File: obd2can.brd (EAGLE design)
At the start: 96.5 x 87.9 mm, 109 parts, among them IC1 SCANTOOL, IC3 LM339PWR, IC4 MCP2551, Q10 BSS138, Q1000 8MHz, Q3 MMBT2222, Q4 MMBT2222, Q7 ZXMP6A13FTA, Q8 MMBT2222, Q9 BSS138, SW1 6X3.5_TACT, U1 3.3V, U1000 SN65HVD235DR, U2 V_REG_317DPACK, U2000 STM32F072-LQFP48, U3 5V Reg., U3000 AP3211KTR-G1, X1000 RJ45_RIGHT_ANGLEMOLEX_95001-2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, X2 Male DB9, X2000 RJ45_RIGHT_ANGLEMOLEX_95001-2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, Y1 16MHz

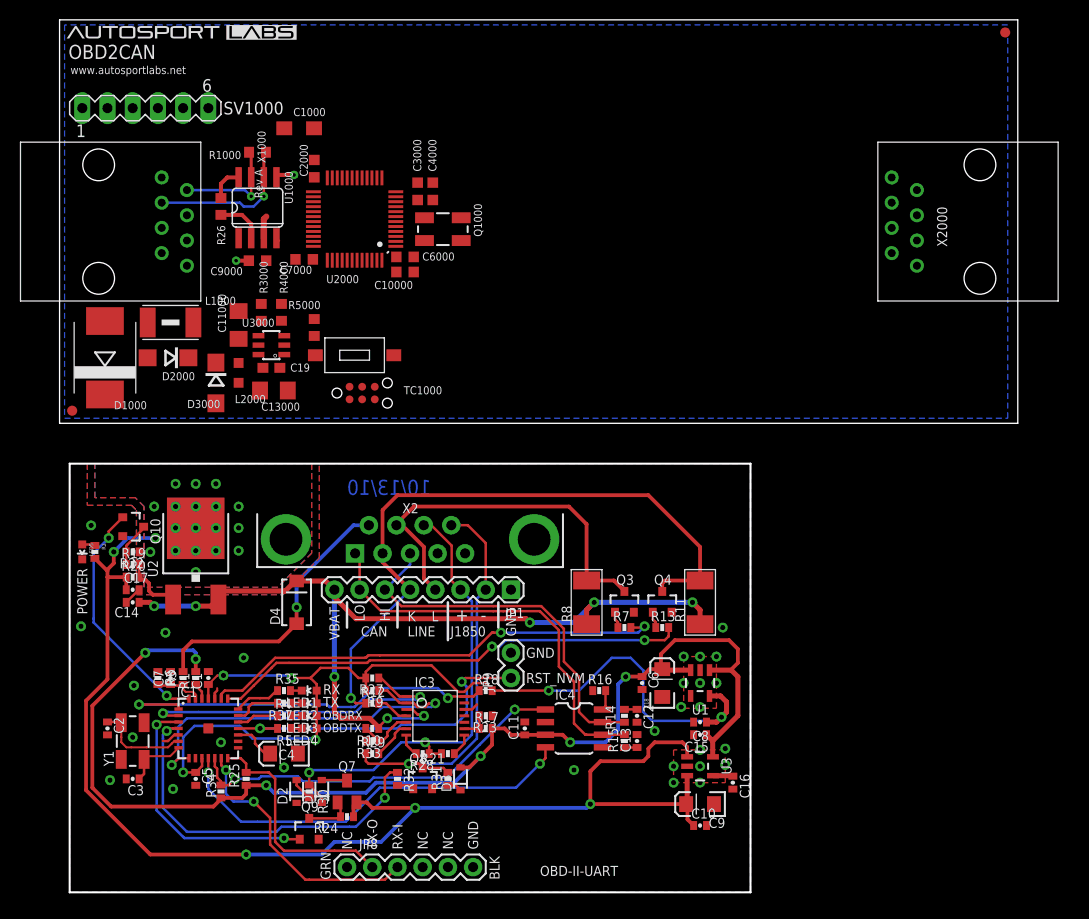
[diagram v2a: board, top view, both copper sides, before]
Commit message: label adjustment, snapshot image
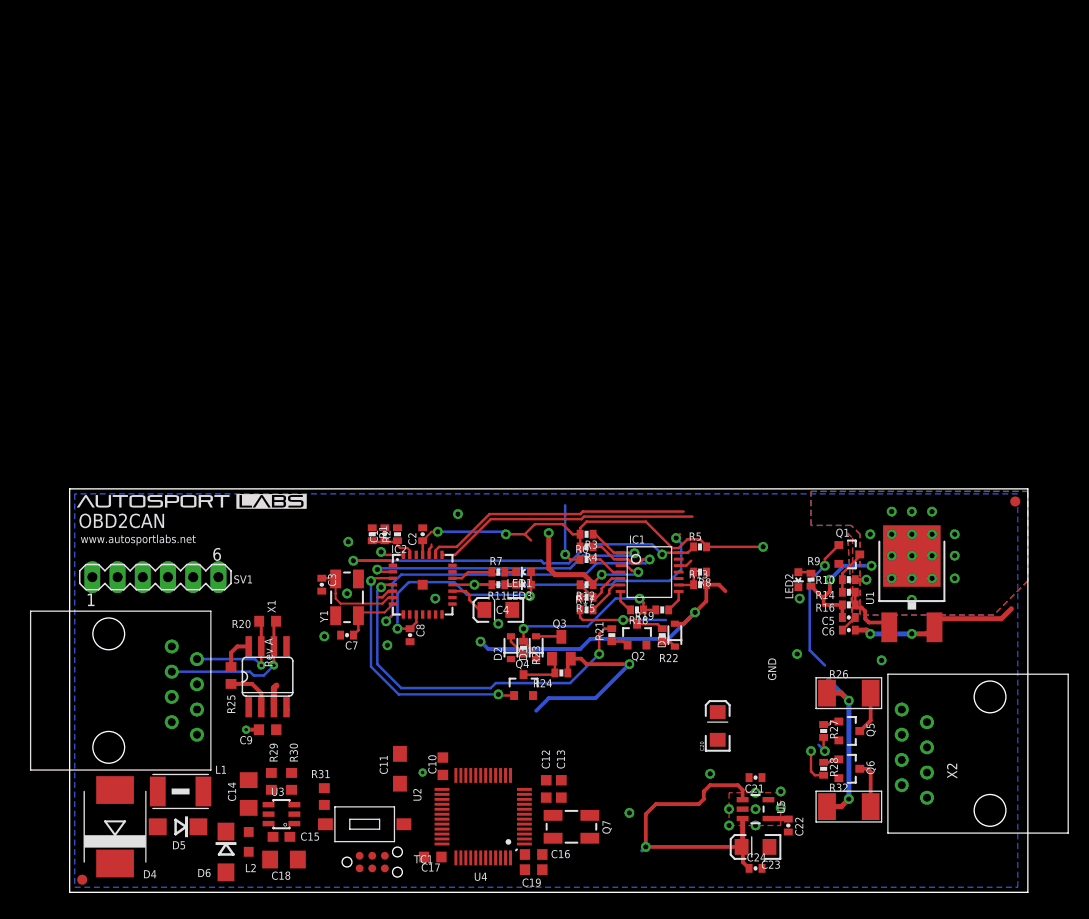
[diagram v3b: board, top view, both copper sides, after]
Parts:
- removed C1000: 10uF, rcl:SMC_A
- removed C10000: 1uf, rcl:C0603K
- removed C11000, C13000: 22uF, rcl:C1206
- removed C2000, C6000, C9000: 0.1uf, rcl:C0603K
- removed C3000, C7000: 4.7uf, rcl:C0603K
- removed C4000: 0.01uf, rcl:C0603K
- removed D1000: (no value), diode:SMC
- removed D2000: 400V 1A, smt_diodes:SMA
- removed D3000: SCHOTTKY, smt_diodes:SMA
- removed IC3: LM339PWR, _stn_logic:TSSOP-14
- removed IC4: MCP2551, _stn_microchip:SO-8
- removed JP1: (no value), SparkFun:1X08
- removed JP8: DNP, SparkFun:FTDI_BASIC
- removed JP9: DNP, SparkFun:1X02
- removed L1000: (no value), wuerth-elektronik:1812
- removed L2000: 4.7uH, rcl:L2012C
- removed LED4, LED5: RED, SparkFun:LED-0603
- removed Q10, Q9: BSS138, SparkFun:SOT23-3
- removed Q1000: 8MHz, SparkFun2:CRYSTAL-SMD-5X3
- removed Q8: MMBT2222, SparkFun:SOT23-3
- removed R1000: 120, rcl:R0603
- removed R3000: 49.9K 1%, rcl:R0603
- removed R33: 10k, SparkFun:0402-RES
- removed R34: 1.5k, SparkFun:0402-RES
- removed R35, R37: 330, SparkFun:0402-RES
- removed R4000: 16.2K 1%, rcl:R0603
- removed R5000: 4.7K, rcl:R0603
- removed SV1000: (no value), con-lstb:MA06-1
- removed TC1000: TC2030-IDC-NL, TagConnect:TC2030-IDC-NL
- removed U1000: SN65HVD235DR, can:SO08
- removed U2000: STM32F072-LQFP48, stm32f0:LQFP48
- removed U3000: AP3211KTR-G1, diodes_inc:SOT-23-6
- removed X1000, X2000: RJ45_RIGHT_ANGLEMOLEX_95001-2881, FCI_RJ12:RJ45_RIGHT_ANGLE_MOLEX_95001-2881
- added C20, C23: 10uF, SparkFun:EIA3216
- added C21: 2.2uF, SparkFun:0402-CAP
- added C22: 470pF, SparkFun:0402-CAP
- added C24: 0.1uF, SparkFun:0402-CAP
- added D5: 400V 1A, smt_diodes:SMA
- added D6: SCHOTTKY, smt_diodes:SMA
- added IC2: SCANTOOL, SparkFun:_STN_SCANTOOL_QFN-28-S
- added L1: (no value), wuerth-elektronik:1812
- added L2: 4.7uH, rcl:L2012C
- added Q1: BSS138, SparkFun:SOT23-3
- added Q2, Q5, Q6: MMBT2222, SparkFun:SOT23-3
- added SV1: (no value), con-lstb:MA06-1
- added TC1: TC2030-IDC-NL, TagConnect:TC2030-IDC-NL
- added U4: STM32F072-LQFP48, stm32f0:LQFP48
- added U5: 5V Reg., SparkFun:SOT23-5
- added X1: RJ45_RIGHT_ANGLEMOLEX_95001-2881, FCI_RJ12:RJ45_RIGHT_ANGLE_MOLEX_95001-2881
- C1, C6: value 1uF -> 0.1uF
- C10: value 0.1uF -> 0.1uf; device SparkFun:0402-CAP -> rcl:C0603K
- C11: value 1uF -> 10uF; device SparkFun:0402-CAP -> rcl:SMC_A
- C12: value 560pF -> 4.7uf; device SparkFun:0402-CAP -> rcl:C0603K
- C13: value 560pF -> 0.01uf; device SparkFun:0402-CAP -> rcl:C0603K
- C14: value 0.1uF -> 22uF; device SparkFun:0402-CAP -> rcl:C1206
- C15: value 2.2uF -> 10nF; device SparkFun:0402-CAP -> rcl:C0603
- C16: value 470pF -> 0.1uf; device SparkFun:0402-CAP -> rcl:C0603K
- C17: value 1uF -> 4.7uf; device SparkFun:0402-CAP -> rcl:C0603K
- C18: value 10uF -> 22uF; device SparkFun:EIA3216 -> rcl:C1206
- C19: value 10nF -> 1uf; device rcl:C0603 -> rcl:C0603K
- C2: value 27pF -> 1uF
- C7: value 0.1uF -> 27pF
- C8: value 4.7uF -> 1uF
- C9: value 10uF -> 0.1uf; device SparkFun:EIA3216 -> rcl:C0603K
- D4: value MBRA140 -> (none); device SparkFun:SMA-DIODE -> diode:SMC
- IC1: value SCANTOOL -> LM339PWR; device SparkFun:_STN_SCANTOOL_QFN-28-S -> _stn_logic:TSSOP-14
- LED3: value YELLOW -> RED
- Q3: value MMBT2222 -> ZXMP6A13FTA; device SparkFun:SOT23-3 -> SparkFun:SOT23
- Q4: value MMBT2222 -> BSS138
- Q7: value ZXMP6A13FTA -> 8MHz; device SparkFun:SOT23 -> SparkFun2:CRYSTAL-SMD-5X3
- R1: value 10k -> 10K
- R10: value 10k -> 374
- R11: value 510 0.5W -> 330; device _stn_rcl:2010 -> SparkFun:0402-RES
- R13: value 1k -> 1.2k
- R14: value 100 -> 866
- R15: value 100 -> 10k
- R16: value 4.7k -> 240
- R17: value 1.2k -> 10k
- R19: value 866 -> 10k
- R2: value 1k -> 62K
- R20: value 240 -> 120; device SparkFun:0402-RES -> rcl:R0603
- R21, R27, R28, R9: value 10k -> 1k
- R22: value 374 -> 10k
- R23: value 4.7k -> 10k
- R25: value 4.7k -> 4.7K; device SparkFun:0402-RES -> rcl:R0603
- R26: value 4.7K -> 510 0.5W; device rcl:R0603 -> _stn_rcl:2010
- R29: value 10k -> 49.9K 1%; device SparkFun:0402-RES -> rcl:R0603
- R3: value 62K -> 10k
- R30: value 10k -> 16.2K 1%; device SparkFun:0402-RES -> rcl:R0603
- R31: value 10k -> 4.7K; device SparkFun:0402-RES -> rcl:R0603
- R32: value 1k -> 510 0.5W; device SparkFun:0402-RES -> _stn_rcl:2010
- R4, R5: value 330 -> 10k
- R6: value 10K -> 10k
- R7: value 1k -> 330
- R8: value 510 0.5W -> 4.7k; device _stn_rcl:2010 -> SparkFun:0402-RES
- U1: value 3.3V -> V_REG_317DPACK; device SparkFun:SOT23-5 -> SparkFun:V-REG_DPACK
- U2: value V_REG_317DPACK -> SN65HVD235DR; device SparkFun:V-REG_DPACK -> can:SO08
- U3: value 5V Reg. -> AP3211KTR-G1; device SparkFun:SOT23-5 -> diodes_inc:SOT-23-6
- X2: value Male DB9 -> RJ45_RIGHT_ANGLEMOLEX_95001-2881; device SparkFun:DB9_MALE -> FCI_RJ12:RJ45_RIGHT_ANGLE_MOLEX_95001-2881
- moved R26 80.0 mm to (78.5, 20.1), turned to 0 degrees
- moved C5 67.8 mm to (78.5, 27.7), turned to 0 degrees
- moved X2 62.3 mm to (92.7, 14.0), turned to 90 degrees
- moved C19 57.0 mm to (46.7, 2.29)
- moved R22 54.0 mm to (59.7, 25.9), turned to 90 degrees
- moved R19 53.5 mm to (59.7, 28.4)
- moved LED2 50.8 mm to (73.4, 31.5), turned to 180 degrees
- moved R10 50.3 mm to (78.5, 31.5)
- moved SW1 47.3 mm to (29.7, 6.86)
- moved IC1 47.2 mm to (58.4, 32.3), turned to 270 degrees
- moved R27 45.8 mm to (75.9, 16.3), turned to 270 degrees
- moved R5 45.7 mm to (63.5, 34.8), turned to 0 degrees
- moved R9 45.6 mm to (74.7, 31.5), turned to 270 degrees
- moved R32 45.6 mm to (78.5, 8.64), turned to 0 degrees
- moved R6 44.8 mm to (52.1, 33.5), turned to 0 degrees
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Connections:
- removed net 3.3V: C1.1, C5.1, C8.1, IC1.10, IC1.25, LED1.A, LED2.A, LED3.A, LED4.A, R18.2, R27.2, R9.2, U1.5
- removed net CAN_HI: IC4.7, JP1.6, R14.2, X2.3
- removed net CAN_LO: IC4.6, JP1.7, R15.2, X2.5
- removed net N$10: C12.1, R14.1
- removed net N$11: IC4.8, R16.2
- removed net N$27: C13.1, R15.1
- removed net N$35: LED1.C, R35.2
- removed net N$36: LED2.C, R37.1
- removed net RX-I: IC1.13, JP8.TXO
- removed net RX-STAT: IC1.21, R35.1
- removed net TX-O: IC1.14, JP8.RXI, R25.2
- removed net TX-STAT: IC1.20, R37.2
- removed net USART2_RX: U2000.13
- removed net USART2_TX: U2000.12
- removed net VBAT: C14.1, D4.C, IC3.3, JP1.8, R10.1, R11.1, R8.1, U2.3
- removed net VBATT_RAW: D4.A, R3.2, X2.9
- new net RESET_STN: IC2.26
- new net RX_FROM_STN: IC2.14, U4.13
- new net TX_TO_STN: IC2.13, U4.12
- net !ISO_K_TX: now also IC2.22, R28.2; no longer IC1.22, R13.2
- net !ISO_L_TX: now also IC2.23, R27.2; no longer IC1.23, R7.2
- net !ISO_RX: now also IC1.2, IC2.8, R4.1; no longer IC1.8, IC3.2, R9.1
- net !OBD_RX_STATUS!/PGC: now also IC2.19, R7.1; no longer IC1.19, R4.1
- net !PWR_SAVE: now also IC2.15; no longer IC1.15
- net !VPW_RX: now also IC1.14, IC2.1, R5.1; no longer IC1.1, IC3.14, R18.1
- net +12V: now also L1.2, R2.2, X1.P8, X2.P8; no longer L1000.2, X1000.P8, X2000.P8
- net +5V: now also SV1.3; no longer SV1000.3
- net 5V: now also C20.A, C21.1, D1.2, R13.2, U5.5; no longer C11.1, C15.1, C18.A, C6.1, D3.2, IC4.3, R1.2, R17.2, R25.1, R34.1, U1.1, U1.3, U3.5
- net AGND: now also U4.8; no longer U2000.8
- net ANALOG_1_ADC: now also U4.10; no longer U2000.10
- net BATT_V: now also C1.1, IC2.27, R1.2, R2.1; no longer C7.1, IC1.27, R3.1, R6.2
- net CANH: now also R20.1, U2.7, X1.P2; no longer R1000.1, U1000.7, X1000.P2
- net CANL: now also R20.2, U2.6, X1.P3; no longer R1000.2, U1000.6, X1000.P3
- net CAN_RX: now also U2.4, U4.32; no longer IC1.11, IC4.4, U1000.4, U2000.32
- net CAN_TX: now also U2.1, U4.33; no longer IC1.12, IC4.1, R34.2, U1000.1, U2000.33
- net GND: now also C11.-, C18.2, C19.2, C20.C, C21.2, C22.2, C23.C, C24.2, C9.2, D4.A, D6.A, IC1.12, IC2.16, IC2.24, IC2.5, IC2.EXP, LED2.C, Q1.2, Q2.2, Q5.2, Q6.2, R1.1, R10.1, R15.2, R25.1, R30.2, R8.1, SV1.1, TC1.5, U2.2, U2.5, U4.23, U4.35, U4.44, U4.47, U5.2, X1.P1, X2.P1; no longer C1000.-, C10000.2, C11.2, C11000.2, C13000.2, C15.2, C18.C, C2000.2, C3000.2, C4000.2, C6000.2, C7000.2, C9.C, C9000.2, D1000.A, D3000.A, IC1.16, IC1.24, IC1.5, IC1.EXP, IC3.12, IC4.2, JP1.1, JP8.GND, JP9.2, LED5.C, Q10.2, Q3.2, Q8.2, Q9.2, R16.1, R22.1, R23.1, R26.1, R33.2, R4000.2, R6.1, SV1000.1, TC1000.5, U1.2, U1000.2, U1000.5, U2000.23, U2000.35, U2000.44, U2000.47, U3000.2, X1000.P1, X2.1, X2.2, X2000.P1
- net HOST_PRESENT: now also IC2.9; no longer IC1.9
- net J1850BUS+: now also D3.1, R18.1, R19.1, R23.1, X2.P4; no longer D1.1, JP1.3, R21.1, R28.1, R30.1, X2.7
- net J1850BUS+_TX: now also IC2.3, Q4.1; no longer IC1.3, Q9.1
- net J1850BUS-: now also Q2.3, R17.1, R22.2, X2.P5; no longer JP1.2, Q8.3, R29.1, R31.2, X2.6
- net J1850BUS-_TX: now also IC2.4, R21.1; no longer IC1.4, R32.1
- net K-LINE: now also Q6.3, R32.2, R6.1, X2.P7; no longer JP1.5, Q4.3, R11.2, R12.1, X2.4
- net L-LINE: now also Q5.3, R26.2, X2.P6; no longer JP1.4, Q3.3, R8.2, X2.8
- net N$1: now also IC1.7, R18.2; no longer IC3.7, R28.2
- net N$12: now also IC1.9, R13.1, R8.2; no longer IC3.9, R17.1, R23.2
- net N$13: now also IC1.4, R6.2; no longer IC3.4, R12.2
- net N$14: now also D1.1, R22.1; no longer D3.1, R31.1
- net N$15: now also R25.2, U2.8; no longer R26.2, U1000.8
- net N$16: now also R29.2, R30.1, U3.3; no longer R3000.2, R4000.1, U3000.3
- net N$17: now also C15.2, U3.1; no longer C19.2, U3000.1
- net N$18: now also Q3.1, Q4.3; no longer Q7.1, Q9.3
- net N$19: now also C15.1, D6.C, L2.1, U3.6; no longer C19.1, D3000.C, L2000.1, U3000.6
- net N$22: now also Q1.3, R10.2, R14.1; no longer Q10.3, R19.1, R22.2
- net N$24: now also R23.2; no longer R30.2
- net N$25: now also Q2.1, R21.2; no longer Q8.1, R32.2
- net N$26: now also IC2.17; no longer IC1.17
- net N$3: now also IC1.6, R17.2; no longer IC3.6, R29.2
- net N$30: now also LED1.C, R7.2; no longer LED3.C, R4.2
- net N$31: now also LED3.C, R11.1; no longer LED4.C, R5.1
- net N$32: now also LED2.A, R9.1; no longer LED5.A, R2.1
- net N$34: now also C22.1, U5.4; no longer C16.1, U3.4
- net N$4: now also Q6.1, R28.1; no longer Q4.1, R13.1
- net N$40: now also Q7.3, U4.6; no longer Q1000.3, U2000.6
- net N$42: now also Q7.1, U4.5; no longer Q1000.1, U2000.5
- net N$5: now also Q5.1, R27.1; no longer Q3.1, R7.1
- net N$50: now also D5.A, L1.1; no longer D2000.A, L1000.1
- net N$6: now also IC1.5, R12.2, R15.1; no longer IC3.5, R10.2, R33.1
- net N$7: now also IC1.8, R19.2; no longer IC3.8, R21.2
- net N$8: now also R14.2, R16.2, U1.1; no longer R19.2, R20.2, U2.1
- net N$9: now also D3.2, Q3.3; no longer D1.2, Q7.3
- net OSC1: now also C3.1, IC2.6; no longer C2.1, IC1.6
- net OSC2: now also C7.1, IC2.7; no longer C3.1, IC1.7
- net PWM/!VPW: now also IC2.28, Q1.1; no longer IC1.28, Q10.1
- net PWM_RX: now also IC1.1, IC2.2, R3.1; no longer IC1.2, IC3.1, R27.1
- net RESET: now also R31.1, TC1.3, U4.7; no longer IC1.26, R1.1, R5000.1, TC1000.3, U2000.7
- net RST_NVM: now also IC2.18, R11.2; no longer IC1.18, JP9.1, R5.2
- net SAFE12V: now also C14.1, C6.1, D4.C, D5.C, IC1.3, R12.1, R26.1, R32.1, U1.3, U3.4, U3.5; no longer C11000.1, D1000.C, D2000.C, U3000.4, U3000.5
- net SWCLK: now also TC1.4, U4.37; no longer TC1000.4, U2000.37
- net SWDIO: now also TC1.2, U4.34; no longer TC1000.2, U2000.34
- net U3: now also R29.1, R31.2, TC1.1; no longer R3000.1, R5000.2, TC1000.1
- net USART1_RX: now also SV1.4, U4.31; no longer SV1000.4, U2000.31
- net USART1_TX: now also SV1.5, U4.30; no longer SV1000.5, U2000.30
- net V+: now also C10.1, C11.+, C12.1, C13.1, C16.1, C17.1, C18.1, C19.1, C2.1, C8.1, C9.1, IC2.10, IC2.25, L2.2, LED1.A, LED3.A, R3.2, R4.2, R5.2, U2.3, U4.1, U4.24, U4.36, U4.48, U4.9; no longer C1000.+, C10000.1, C13000.1, C2000.1, C3000.1, C4000.1, C6000.1, C7000.1, C9000.1, L2000.2, U1000.3, U2000.1, U2000.24, U2000.36, U2000.48, U2000.9
- net VCC: now also C23.A, C24.1, C5.1, Q3.2, R16.1, R9.2, U1.4, U5.1, U5.3; no longer C10.1, C17.1, C9.A, Q7.2, R2.2, R20.1, U2.4, U3.1, U3.3
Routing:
- net 3.3V: track 98.1 -> 0.00 mm, vias 6 -> 0
- net 5V: track 124.3 -> 31.7 mm, vias 6 -> 2
- net VBAT: track 90.1 -> 0.00 mm, vias 8 -> 0
- net VCC: track 129.3 -> 63.2 mm, vias 22 -> 21
- net V+: track 2.29 -> 67.9 mm, vias 0 -> 5
- net K-LINE: track 67.2 -> 11.4 mm
- net SAFE12V: track 0.00 -> 51.1 mm, vias 0 -> 7
- net CAN_RX: track 42.5 -> 0.36 mm, vias 2 -> 0
- net CAN_LO: track 41.3 -> 0.00 mm
- net CAN_TX: track 39.3 -> 0.00 mm, vias 2 -> 0
- net CAN_HI: track 38.4 -> 0.00 mm
- net L-LINE: track 39.2 -> 4.29 mm
- net VBATT_RAW: track 29.2 -> 0.00 mm, vias 1 -> 0
- net J1850BUS+: track 47.7 -> 19.1 mm
- net J1850BUS-: track 41.7 -> 13.8 mm
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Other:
- board size 96.5 x 87.9 mm -> 96.5 x 40.6 mm
- board text removed: "+"
- board text removed: "-"
- board text removed: "10/13/10"
- board text removed: "BLK"
- board text removed: "CAN"
- board text removed: "GRN"
- board text removed: "HI"
- board text removed: "J1850"
- board text removed: "K"
- board text removed: "L"
- board text removed: "LINE"
- board text removed: "LO"
- board text removed: "NC"
- board text removed: "OBD-II-UART"
- board text removed: "OBDRX"
- board text removed: "OBDTX"
- board text removed: "POWER"
- board text removed: "RST_NVM"
- board text removed: "RX"
- board text removed: "RX-I"
- board text removed: "TX"
- board text removed: "TX-O"
- board text removed: "VBAT"
